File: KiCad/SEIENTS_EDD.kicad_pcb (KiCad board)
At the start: 2 copper layers, 148.3 x 117.1 mm, 99 parts, among them IC1 A3144EUA, J1 Conn_01x02_Pin, J201 Screw_Terminal_01x04, J3 Screw_Terminal_01x05, J4 Screw_Terminal_01x02, J7 DE9_Socket, J8 DE9_Pins, M4 Motor_DC, M5 Motor_DC, M6 Motor_DC, Q201 IRLZ44N, SW10 SW_Push, SW11 SW_Push, SW12 SW_Push, SW13 SW_Push, SW14 SW_Push, SW15 SW_Push, SW8 SW_Push, SW9 SW_Push, U1 LM2596S-5, U11 MAX3232, U2 LM1117DT-3.3, U3 MCP2562-E-SN, U4 TMP102xxDRL, U5 TB6612FNG, U6 24LC256, U67 PIC24HJ64GP504-I/PT, U7 ATtiny1616-M, U8 DRV8871DDA, Y1 8 MHz

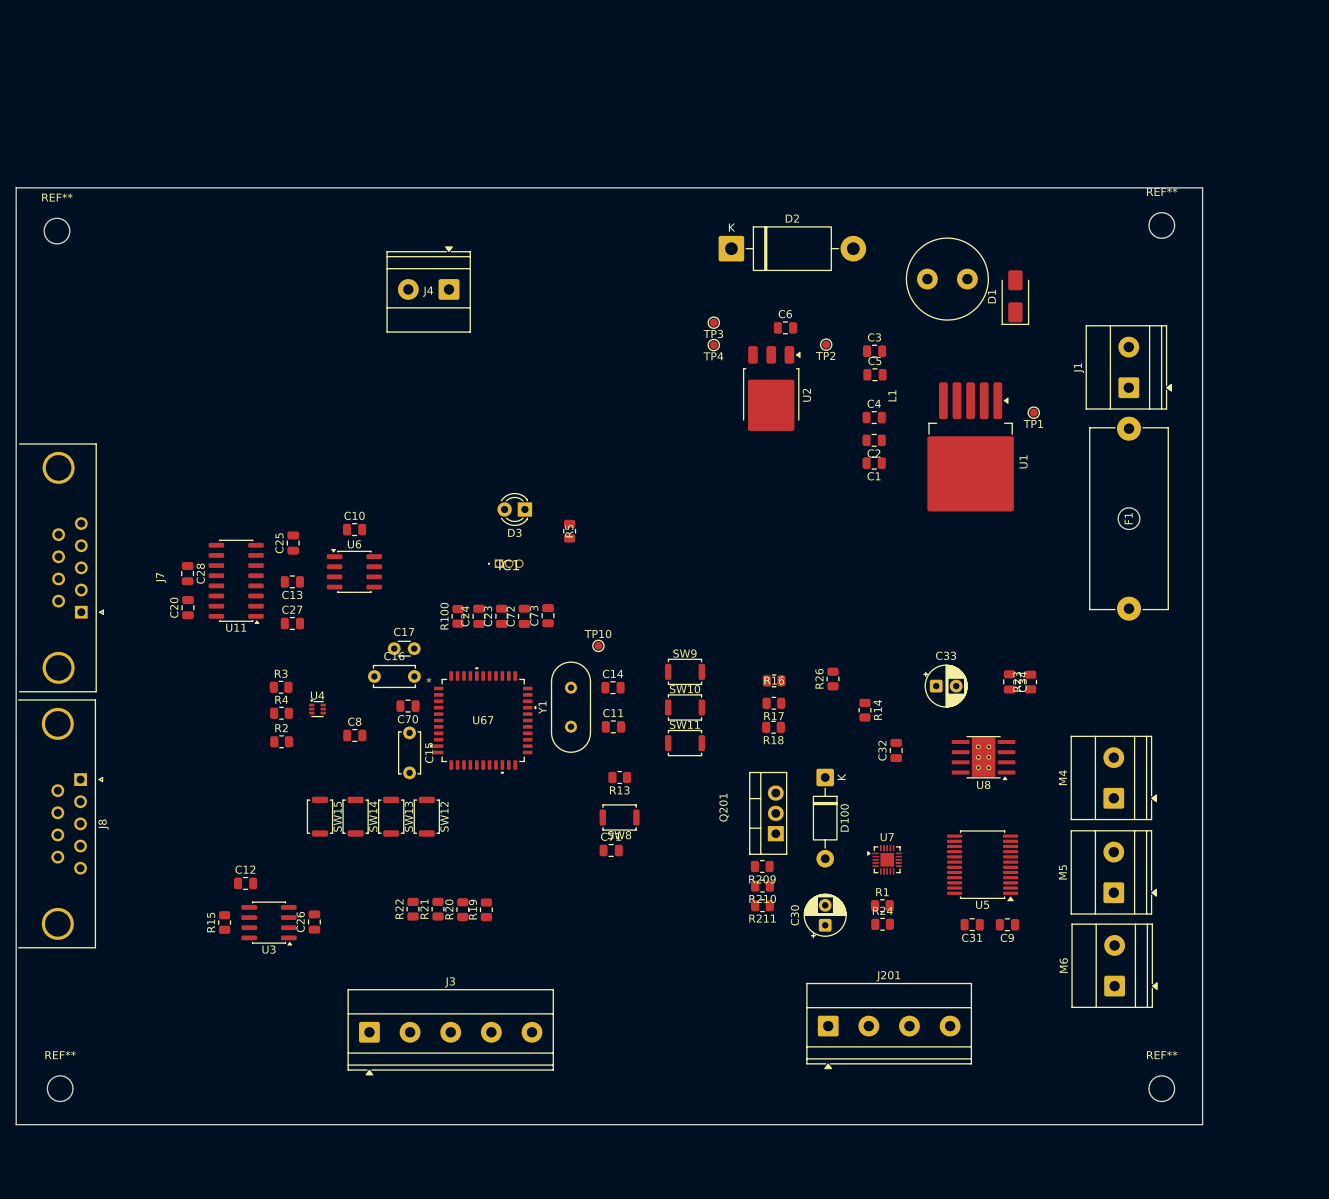
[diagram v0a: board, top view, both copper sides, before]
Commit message: Modificació al placement
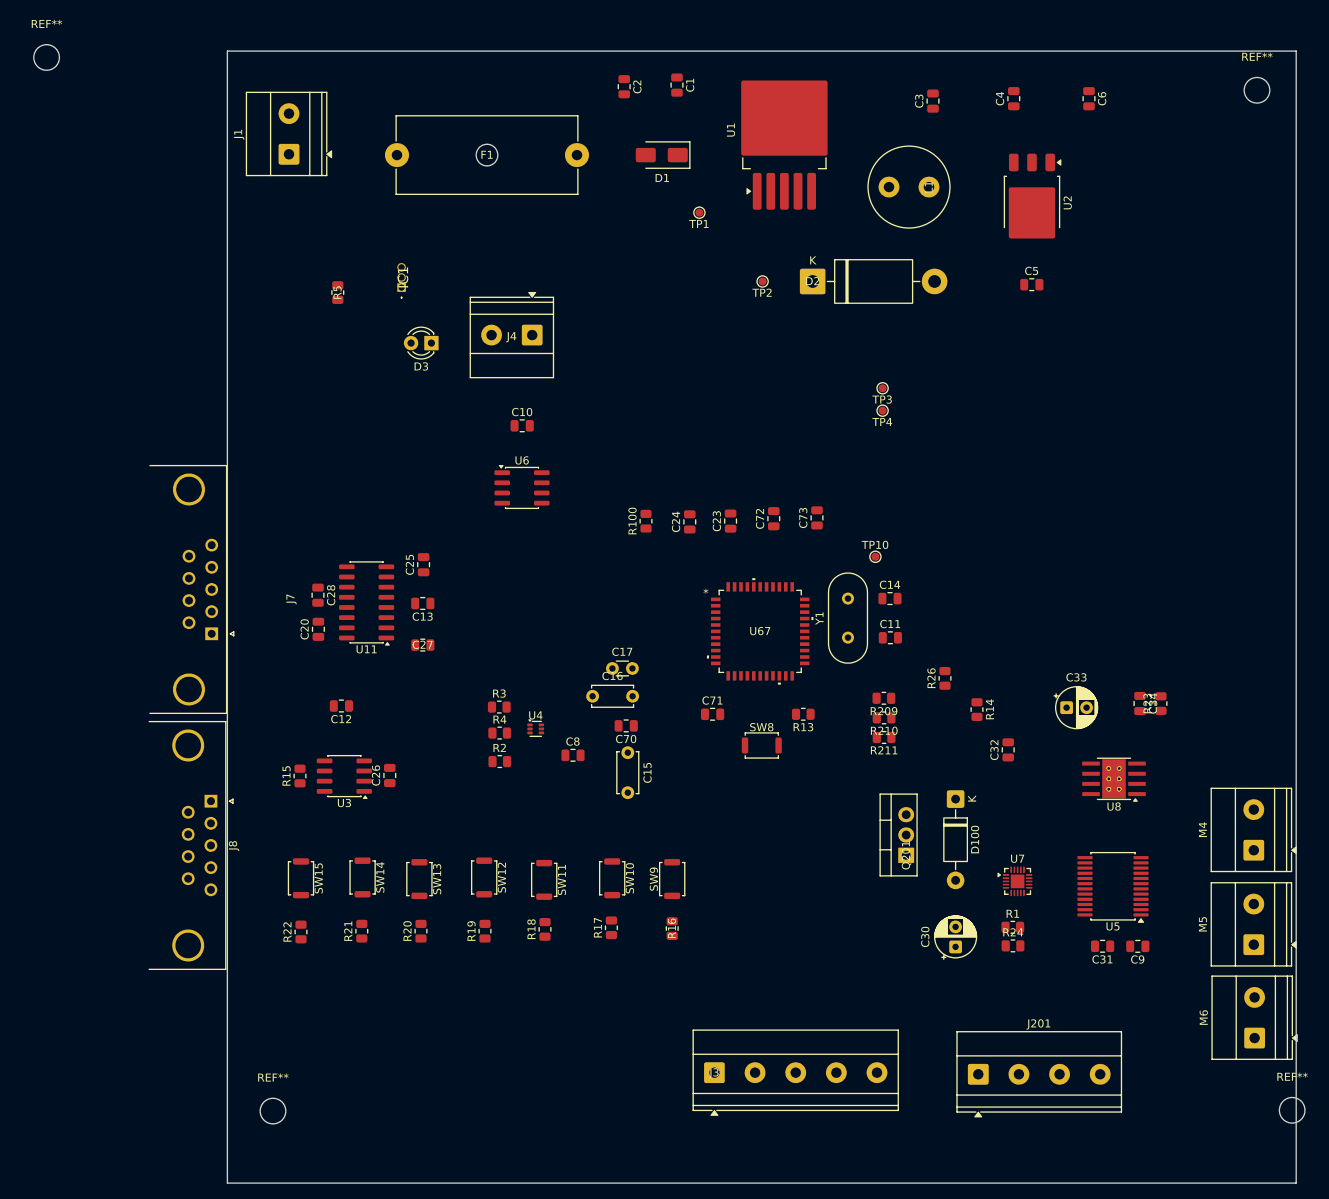
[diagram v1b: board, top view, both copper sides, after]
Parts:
- moved J1 109.0 mm to (124.0, 32.1)
- moved F1 107.6 mm to (137.5, 32.2), turned to 0 degrees
- moved C2 54.1 mm to (165.9, 23.6), turned to -90 degrees
- moved C1 53.3 mm to (172.5, 23.4), turned to -90 degrees
- moved TP1 48.7 mm to (175.3, 39.4)
- moved D1 47.6 mm to (170.6, 32.2), turned to 180 degrees
- moved U1 47.6 mm to (185.9, 29.1), turned to 90 degrees
- moved C6 47.6 mm to (224.0, 25.1), turned to -90 degrees
- moved C4 43.5 mm to (214.6, 25.1), turned to 90 degrees
- moved J3 43.4 mm to (177.2, 146.9)
- moved R5 41.6 mm to (130.1, 49.4)
- moved U2 40.5 mm to (216.9, 38.2)
- moved R18 38.1 mm to (156.0, 129.0), turned to 90 degrees
- moved IC1 36.6 mm to (138.1, 48.8), turned to 90 degrees
- moved C11 36.4 mm to (199.2, 92.5)
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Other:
- board size 148.3 x 117.1 mm -> 133.6 x 141.5 mm
